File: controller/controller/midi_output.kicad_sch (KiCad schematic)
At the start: 5 parts, among them J11-O1 SJ-3524-SMT

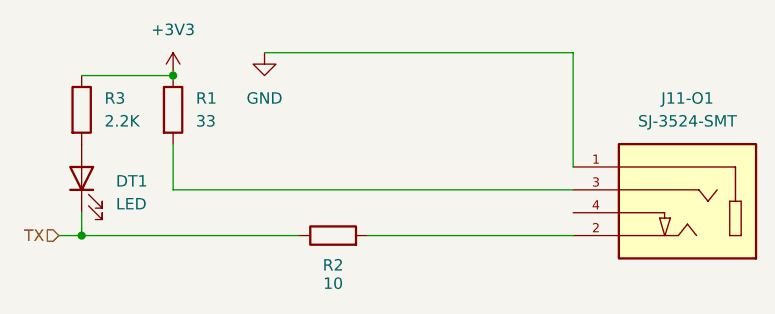
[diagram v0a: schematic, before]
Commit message: update to v2
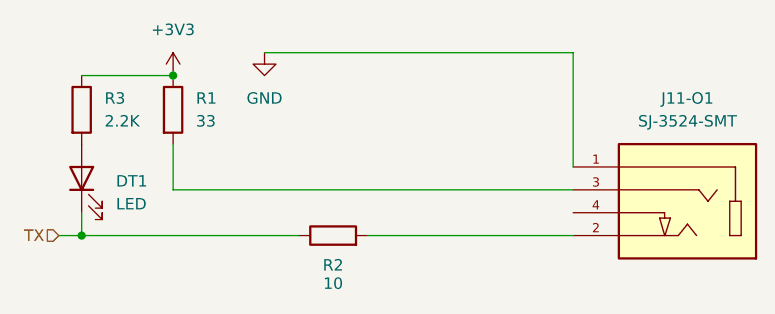
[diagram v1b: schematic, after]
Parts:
- J11-O1: footprint SJ-3524-SMT:CUI_SJ-3524-SMT -> MIDI_projects:CUI_SJ-3524-SMT
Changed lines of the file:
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@@
 	(wire
 		(pts
-			(xy 100.33 100.33) (xy 100.33 95.25)
+			(xy 100.33 95.25) (xy 100.33 100.33)
 		)
 		(stroke
@@
 	(wire
 		(pts
+			(xy 110.49 85.09) (xy 144.78 85.09)
+		)
+		(stroke
+			(width 0)
+			(type default)
+		)
+	)
+	(wire
+		(pts
+			(xy 90.17 105.41) (xy 114.3 105.41)
+		)
+		(stroke
+			(width 0)
+			(type default)
+		)
+	)
+	(wire
+		(pts
+			(xy 100.33 100.33) (xy 144.78 100.33)
+		)
+		(stroke
+			(width 0)
+			(type default)
+		)
+	)
+	(wire
+		(pts
+			(xy 90.17 105.41) (xy 90.17 102.87)
+		)
+		(stroke
+			(width 0)
+			(type default)
+		)
+	)
+	(wire
+		(pts
+			(xy 144.78 85.09) (xy 144.78 97.79)
+		)
+		(stroke
+			(width 0)
+			(type default)
+		)
+	)
+	(wire
+		(pts
 			(xy 121.92 105.41) (xy 144.78 105.41)
-		)
-		(stroke
-			(width 0)
-			(type default)
-		)
-	)
-	(wire
-		(pts
-			(xy 110.49 85.09) (xy 144.78 85.09)
-		)
-		(stroke
-			(width 0)
-			(type default)
-		)
-	)
-	(wire
-		(pts
-			(xy 90.17 105.41) (xy 114.3 105.41)
-		)
-		(stroke
-			(width 0)
-			(type default)
-		)
-	)
-	(wire
-		(pts
-			(xy 90.17 105.41) (xy 90.17 102.87)
-		)
-		(stroke
-			(width 0)
-			(type default)
-		)
-	)
-	(wire
-		(pts
-			(xy 100.33 100.33) (xy 144.78 100.33)
-		)
-		(stroke
-			(width 0)
-			(type default)
-		)
-	)
-	(wire
-		(pts
-			(xy 144.78 85.09) (xy 144.78 97.79)
 		)
 		(stroke
@@
 			)
 		)
-		(property "Footprint" "SJ-3524-SMT:CUI_SJ-3524-SMT"
+		(property "Footprint" "MIDI_projects:CUI_SJ-3524-SMT"
 			(at 155.194 92.71 0)
 			(effects
@@
 		(lib_id "power:GND")
 		(at 110.49 85.09 0)
+		(mirror y)
 		(unit 1)
 		(exclude_from_sim no)
@@
 		(on_board yes)
 		(dnp no)
-		(fields_autoplaced yes)
 		(property "Reference" "#PWR010"
 			(at 110.49 91.44 0)
